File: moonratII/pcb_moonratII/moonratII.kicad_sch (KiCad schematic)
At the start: 49 parts, among them J1 Barrel_Jack_Switch_SMT, J10 Conn_02x05_Odd_Even, J11 Screw_Terminal_01x02, J2 HS96L03W2C03_0.96_Oled, J5 Conn_02x05_Odd_Even, J6 Screw_Terminal_01x06, J9 Screw_Terminal_01x06, Q1 IRF520N, Q2 BSS138, SW1 6mm 2 Pin Tact NO Breadboard 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, SW2 6mm 2 Pin Tact NO Breadboard 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, SW3 6mm 2 Pin Tact NO Breadboard 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, U1 TMP36GRTZ-REEL7

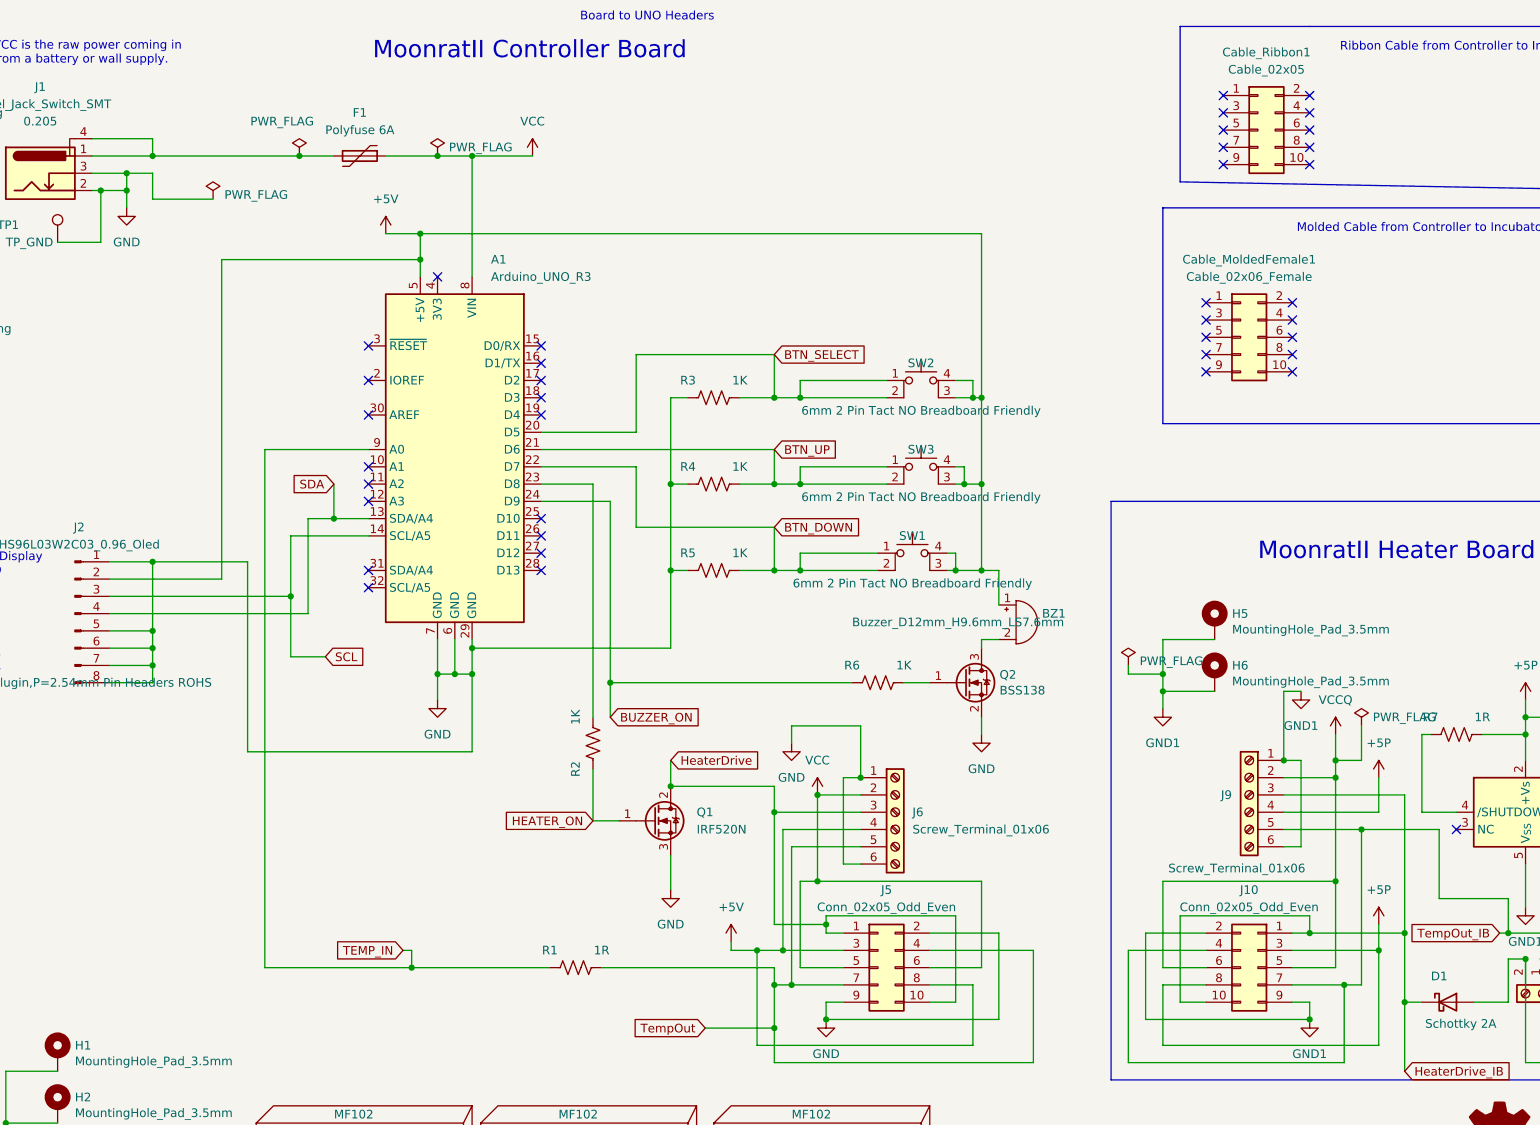
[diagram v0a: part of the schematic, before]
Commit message: Increase size on Heater traces.
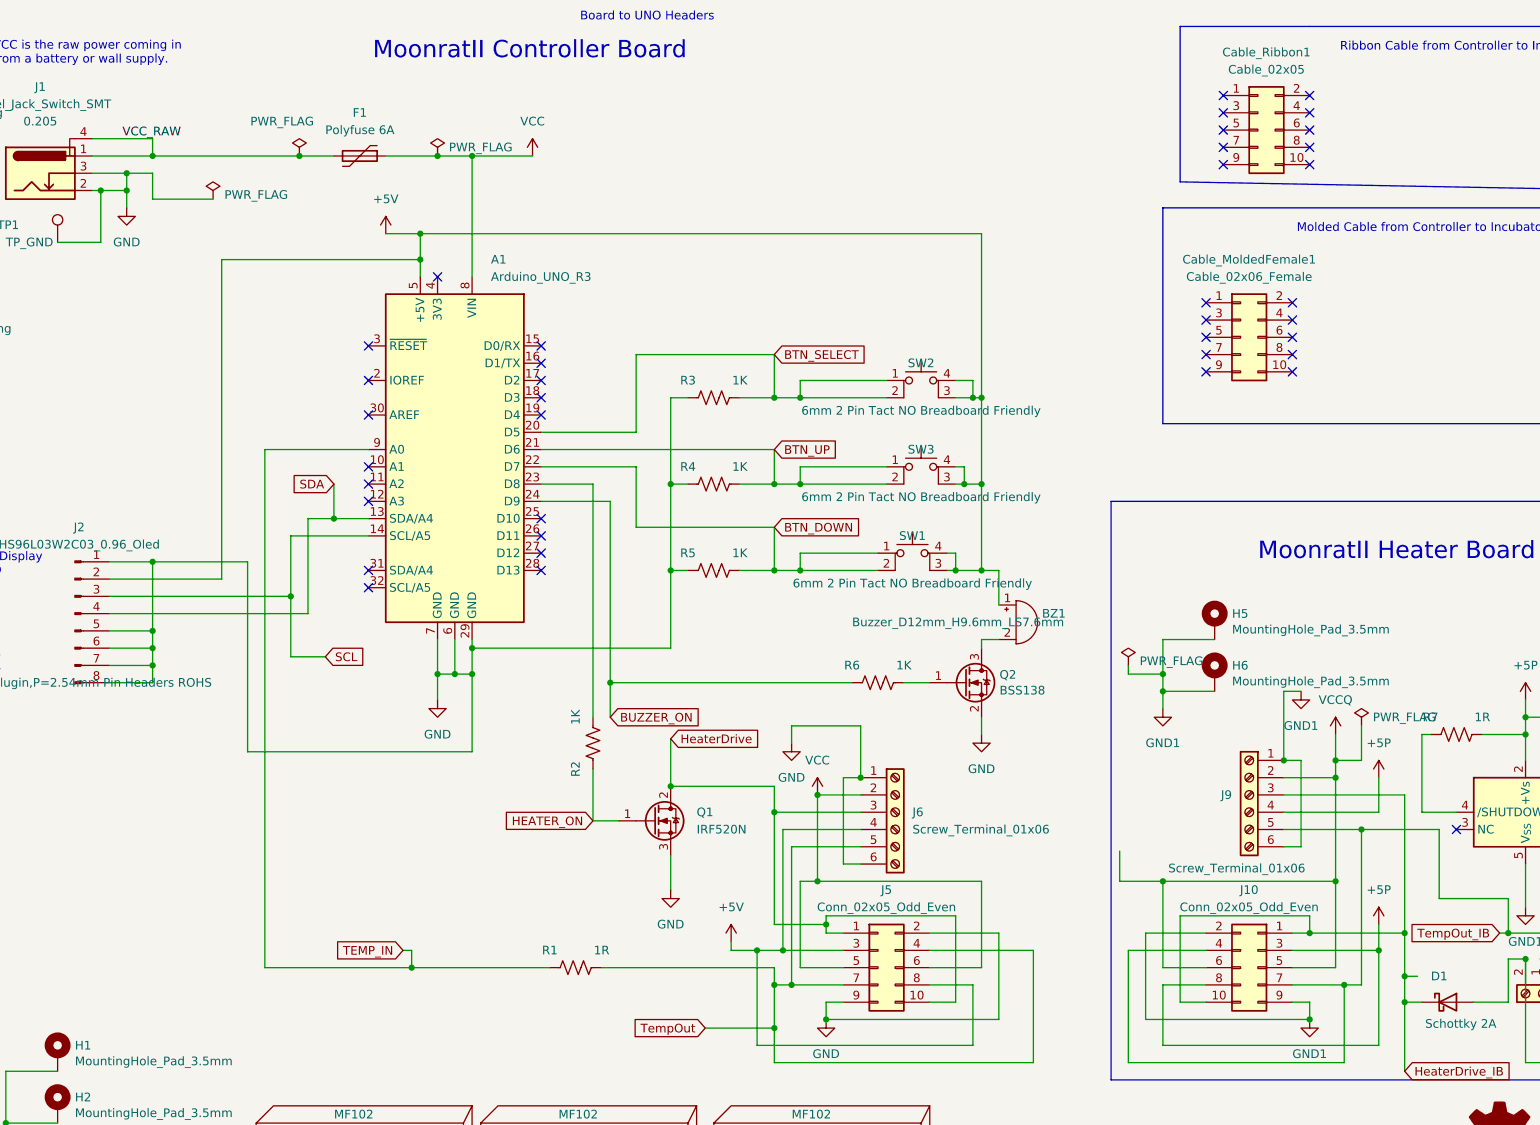
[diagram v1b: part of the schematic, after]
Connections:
- net VCC_RAW: now reaches F1.2, J1.1, J1.4
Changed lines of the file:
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@@
   (title_block
     (title "MoonratII")
-    (date "2023-11-20")
-    (rev "1.0")
+    (date "2024-02-06")
+    (rev "2.0")
     (company "PublicInvention")
     (comment 1 "GNU Affero General Public License v3.0")
@@
   (junction (at 190.5 113.03) (diameter 0) (color 0 0 0 0)
   )
+  (junction (at 190.5 140.97) (diameter 0) (color 0 0 0 0)
+  )
   (junction (at 20.32 191.77) (diameter 0) (color 0 0 0 0)
   )
@@
   (junction (at 130.81 151.13) (diameter 0) (color 0 0 0 0)
   )
+  (junction (at 226.06 154.94) (diameter 0) (color 0 0 0 0)
+  )
   (junction (at 133.35 69.85) (diameter 0) (color 0 0 0 0)
   )
@@
     (stroke (width 0) (type default))
   )
-  (wire (pts (xy 226.06 148.59) (xy 226.06 158.75))
+  (wire (pts (xy 226.06 148.59) (xy 226.06 154.94))
     (stroke (width 0) (type default))
   )
@@
     (stroke (width 0) (type default))
   )
+  (wire (pts (xy 226.06 154.94) (xy 226.06 158.75))
+    (stroke (width 0) (type default))
+  )
   (wire (pts (xy 212.09 158.75) (xy 209.55 158.75))
     (stroke (width 0) (type default))
@@
     (stroke (width 0) (type default))
   )
+  (wire (pts (xy 226.06 154.94) (xy 227.965 154.94))
+    (stroke (width 0) (type default))
+  )
   (wire (pts (xy 190.5 165.1) (xy 222.25 165.1))
     (stroke (width 0) (type default))
@@
     (stroke (width 0) (type default))
   )
+  (wire (pts (xy 184.15 136.525) (xy 184.15 140.97))
+    (stroke (width 0) (type default))
+  )
   (wire (pts (xy 163.83 105.41) (xy 166.37 105.41))
     (stroke (width 0) (type default))
@@
     (stroke (width 0) (type default))
   )
+  (wire (pts (xy 184.15 140.97) (xy 190.5 140.97))
+    (stroke (width 0) (type default))
+  )
   (wire (pts (xy 99.06 80.01) (xy 113.03 80.01))
     (stroke (width 0) (type default))
   )
-  (wire (pts (xy 118.11 123.19) (xy 118.11 127))
+  (wire (pts (xy 118.11 120.015) (xy 118.11 127))
     (stroke (width 0) (type default))
   )
@@
     (effects (font (size 2.54 2.54)) (justify left bottom))
   )
-  (global_label "HeaterDrive" (shape input) (at 118.11 123.19 0) (fields_autoplaced)
+  (label "VCC_RAW" (at 37.465 31.75 0) (fields_autoplaced)
+    (effects (font (size 1.27 1.27)) (justify left bottom))
+  )
+  (global_label "HeaterDrive" (shape input) (at 118.11 120.015 0) (fields_autoplaced)
     (effects (font (size 1.27 1.27)) (justify left))
-    (property "Intersheetrefs" "${INTERSHEET_REFS}" (at 131.4088 123.1106 0)
+    (property "Intersheetrefs" "${INTERSHEET_REFS}" (at 131.4088 119.9356 0)
       (effects (font (size 1.27 1.27)) (justify left) hide)
     )
@@
     )
   )
+  (netclass_flag "" (length 2.54) (shape round) (at 227.965 154.94 0) (fields_autoplaced)
+    (effects (font (size 1.27 1.27)) (justify left bottom))
+    (property "Netclass" "Heater" (at 228.6635 152.4 0)
+      (effects (font (size 1.27 1.27) italic) (justify left))
+    )
+  )
+  (netclass_flag "" (length 2.54) (shape round) (at 46.99 34.29 0) (fields_autoplaced)
+    (effects (font (size 1.27 1.27)) (justify left bottom))
+    (property "Netclass" "Heater" (at 47.6885 31.75 0)
+      (effects (font (size 1.27 1.27) italic) (justify left))
+    )
+  )
+  (netclass_flag "" (length 2.54) (shape round) (at 247.65 167.64 0) (fields_autoplaced)
+    (effects (font (size 1.27 1.27)) (justify left bottom))
+    (property "Netclass" "Heater" (at 248.3485 165.1 0)
+      (effects (font (size 1.27 1.27) italic) (justify left))
+    )
+  )
+  (netclass_flag "" (length 2.54) (shape round) (at 184.15 136.525 0) (fields_autoplaced)
+    (effects (font (size 1.27 1.27)) (justify left bottom))
+    (property "Netclass" "Heater" (at 184.8485 133.985 0)
+      (effects (font (size 1.27 1.27) italic) (justify left))
+    )
+  )
+  (netclass_flag "" (length 2.54) (shape round) (at 125.73 127 0) (fields_autoplaced)
+    (effects (font (size 1.27 1.27)) (justify left bottom))
+    (property "Netclass" "Heater" (at 126.4285 124.46 0)
+      (effects (font (size 1.27 1.27) italic) (justify left))
+    )
+  )
+  (netclass_flag "" (length 2.54) (shape round) (at 78.74 34.29 0) (fields_autoplaced)
+    (effects (font (size 1.27 1.27)) (justify left bottom))
+    (property "Netclass" "Heater" (at 79.4385 31.75 0)
+      (effects (font (size 1.27 1.27) italic) (justify left))
+    )
+  )
